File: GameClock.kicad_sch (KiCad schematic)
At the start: 2 parts, among them J1 USB_B_Micro, U1 ATmega328P-A

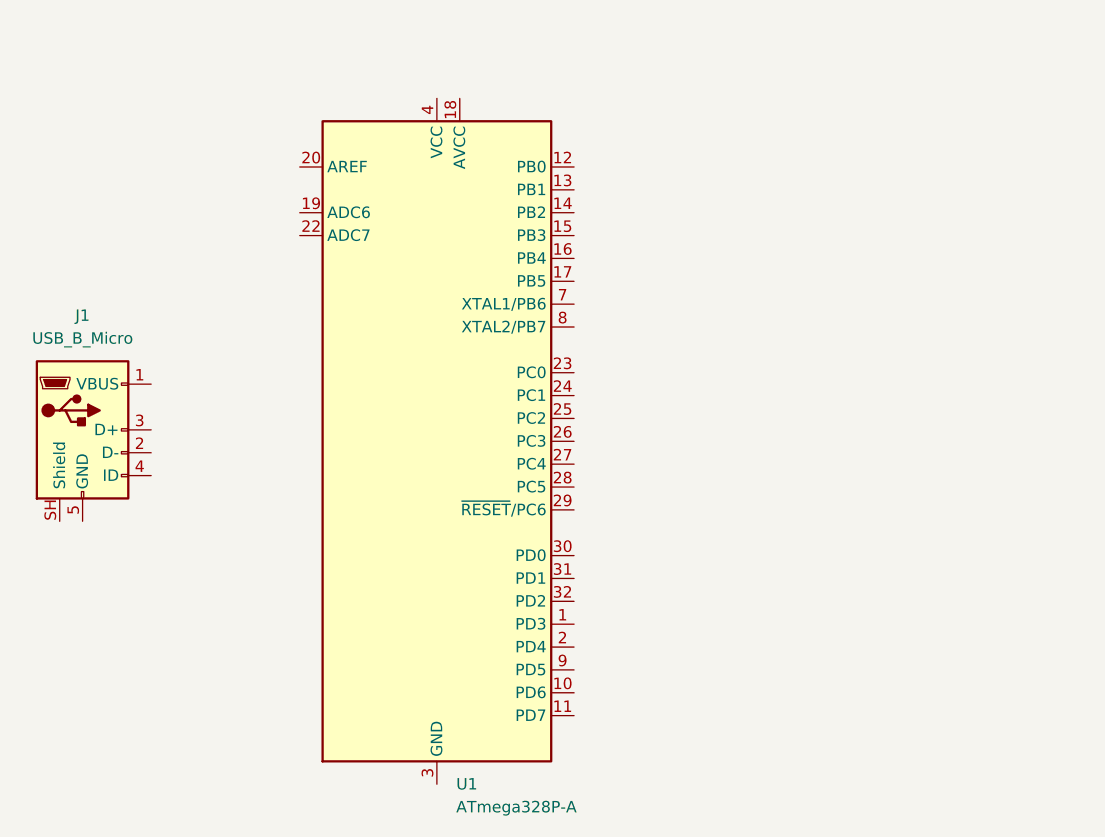
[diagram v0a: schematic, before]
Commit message: finished schema
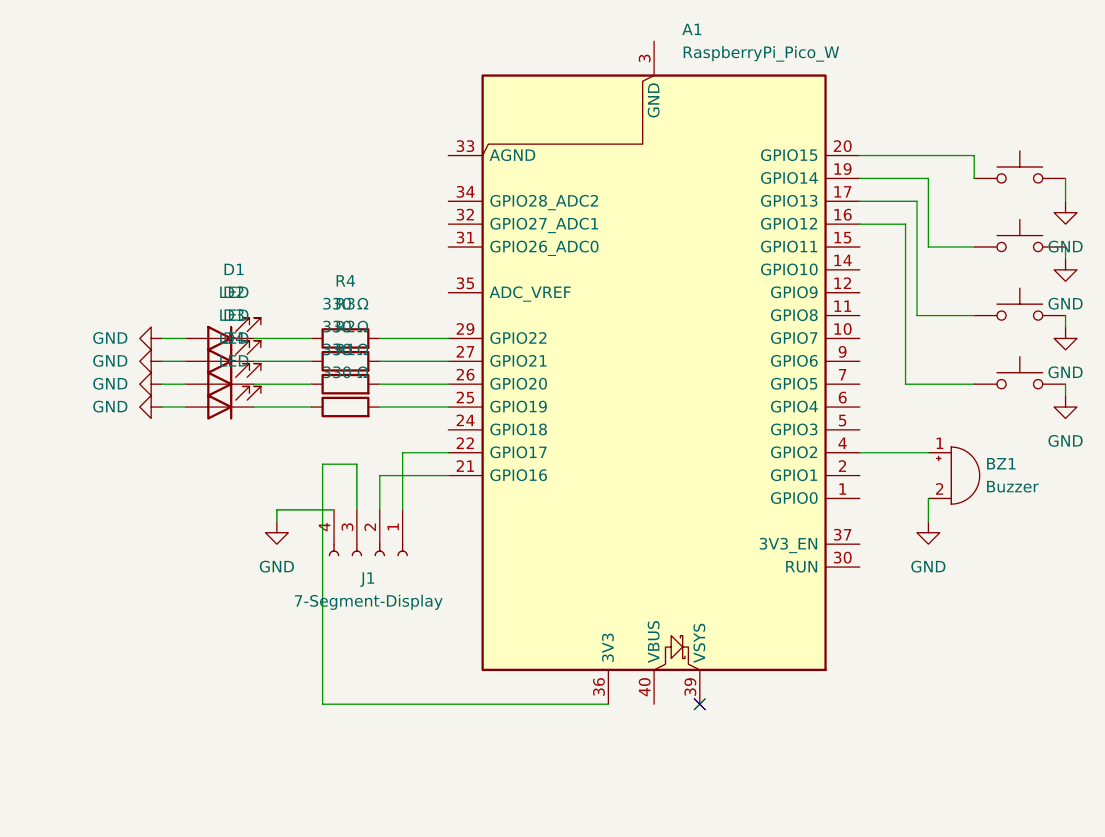
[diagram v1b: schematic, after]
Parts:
- removed J1: USB_B_Micro, symbol Connector:USB_B_Micro
- removed U1: ATmega328P-A, Package_QFP:TQFP-32_7x7mm_P0.8mm, symbol MCU_Microchip_ATmega:ATmega328P-A
- added A1: RaspberryPi_Pico_W, Module:RaspberryPi_Pico_W_SMD_HandSolder, symbol MCU_Module:RaspberryPi_Pico_W
- added BZ1: Buzzer, Buzzer_Beeper:Buzzer_12x9.5RM7.6, symbol Device:Buzzer
- added D1, D2, D3, D4: LED, LED_THT:LED_D2.0mm_W4.0mm_H2.8mm_FlatTop, symbol Device:LED
- added J1: 7-Segment-Display, Connector_PinHeader_2.54mm:PinHeader_1x04_P2.54mm_Vertical, symbol Connector:Conn_01x04_Socket
- added R1, R2, R3, R4: 330 Ω, Resistor_THT:R_Axial_DIN0207_L6.3mm_D2.5mm_P7.62mm_Horizontal, symbol Device:R
- added SW1, SW2, SW3, SW4: SW_Push, Button_Switch_THT:SW_PUSH_6mm, symbol Switch:SW_Push
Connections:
- new net: A1.13 (GND), A1.18 (GND), A1.23 (GND), A1.28 (GND), A1.3 (GND), A1.38 (GND), A1.8 (GND)
- new net: A1.16 (GPIO12), SW4.1
- new net: A1.17 (GPIO13), SW3.1
- new net: A1.19 (GPIO14), SW2.1
- new net: A1.20 (GPIO15), SW1.1
- new net: A1.21 (GPIO16), J1.2 (Pin_2)
- new net: A1.22 (GPIO17), J1.1 (Pin_1)
- new net: A1.25 (GPIO19), R1.2
- new net: A1.26 (GPIO20), R2.2
- new net: A1.27 (GPIO21), R3.2
- new net: A1.29 (GPIO22), R4.2
- new net: A1.36 (3V3), J1.3 (Pin_3)
- new net: A1.4 (GPIO2), BZ1.1 (+)
- new net: D4.1 (K), R1.1
- new net: D1.1 (K), R4.1
- new net: D2.1 (K), R3.1
- new net: D3.1 (K), R2.1
- new net GND: BZ1.2 (-), D1.2 (A), D2.2 (A), D3.2 (A), D4.2 (A), J1.4 (Pin_4), SW1.2, SW2.2, SW3.2, SW4.2
- no-connect marks 0 -> 1
